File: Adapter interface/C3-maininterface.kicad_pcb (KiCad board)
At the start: 4 copper layers, 19.4 x 34.6 mm, 4 parts, among them J1 SFM-120-02-L-DH, J2 SFM-120-02-L-DH

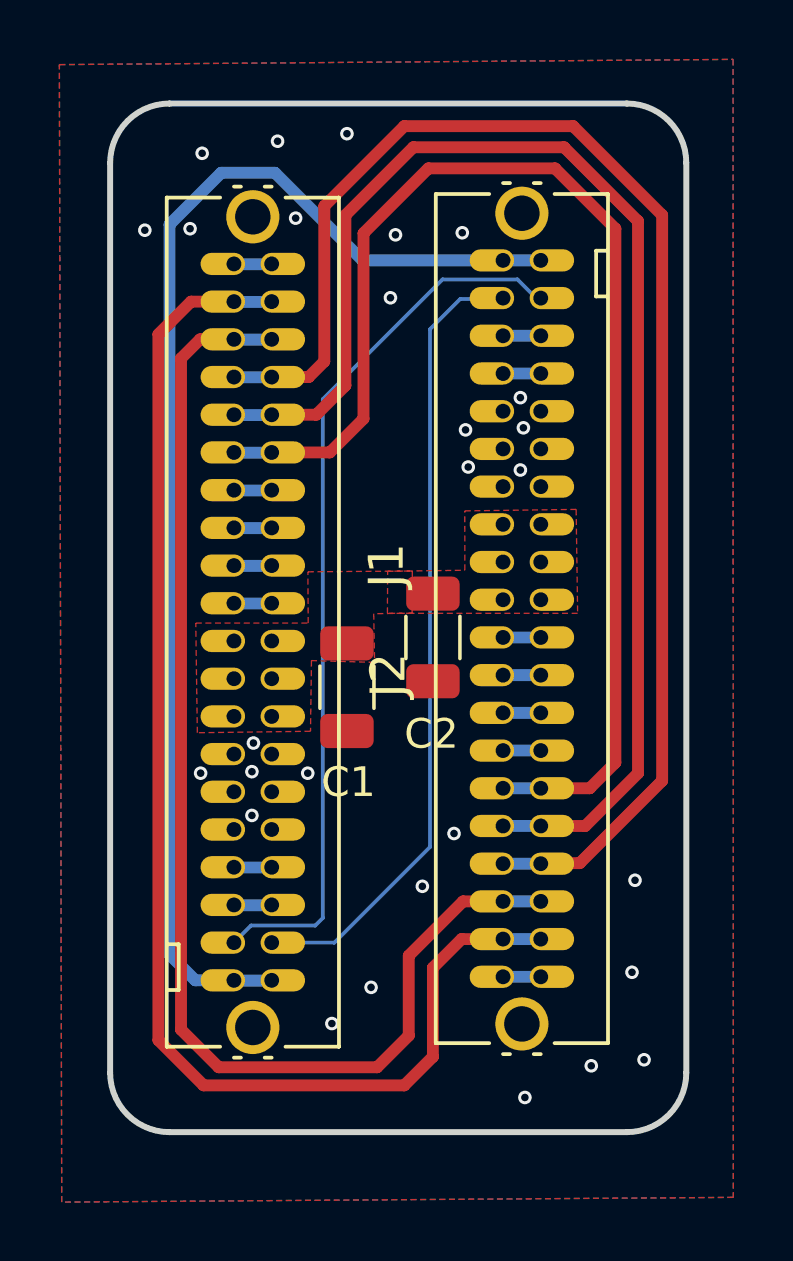
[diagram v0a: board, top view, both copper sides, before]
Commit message: New connectors
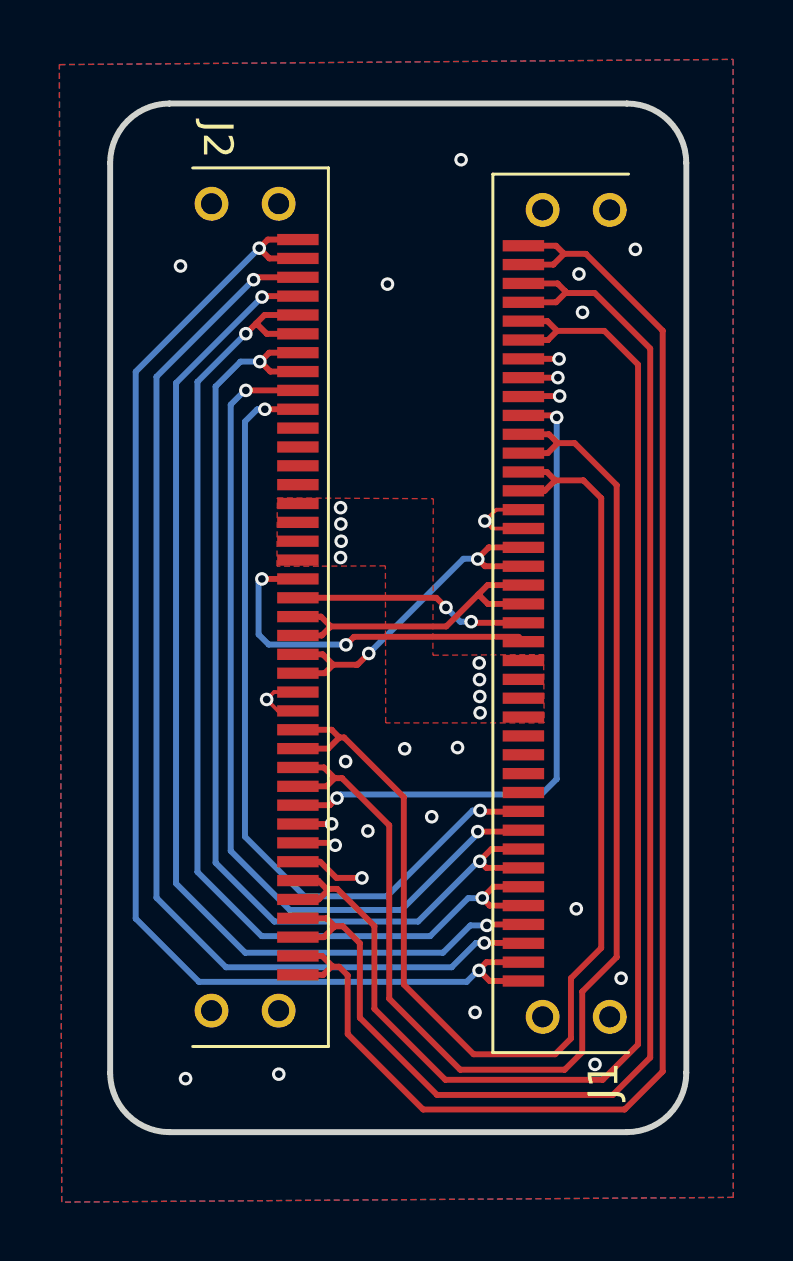
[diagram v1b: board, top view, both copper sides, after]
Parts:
- removed C1, C2: 10u 25V, Capacitor_SMD:C_1206_3216Metric
- J1, J2: footprint oresat-connectors:J-SAMTEC-SFM-120-X1-XXX-D -> oresat-connectors:SFM-120-02-X-DH
- moved J1 4.11 mm to (161.4, 85.6)
- moved J2 2.58 mm to (145.7, 85.4)
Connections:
- J1 pad 10: TURNSTILE-DEPLOY -> SPARE10
- J1 pad 21: VBUS -> SPARE21
- J1 pad 22: VBUS -> SPARE22
- J1 pad 31: GND -> SPARE31
- J1 pad 32: GND -> SPARE32
- J1 pad 7: HELICAL-DEPLOY -> SPARE07
- J1 pad 8: HELICAL-DEPLOY -> SPARE08
- J1 pad 9: TURNSTILE-DEPLOY -> SPARE09
- J2 pad 10: TURNSTILE-DEPLOY -> SPARE10
- J2 pad 21: VBUS -> SPARE21
- J2 pad 22: VBUS -> SPARE22
- J2 pad 31: GND -> SPARE31
- J2 pad 32: GND -> SPARE32
- J2 pad 7: HELICAL-DEPLOY -> SPARE07
- J2 pad 8: HELICAL-DEPLOY -> SPARE08
- J2 pad 9: TURNSTILE-DEPLOY -> SPARE09
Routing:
- net HELICAL-DEPLOY: track 47.8 -> 0.00 mm
- net TURNSTILE-DEPLOY: track 45.6 -> 0.00 mm
- net SPARE07: track 0.00 -> 29.7 mm, vias 0 -> 2
- net SPARE32: track 0.00 -> 29.3 mm, vias 0 -> 2
- net SPARE31: track 0.00 -> 27.4 mm, vias 0 -> 2
- net SPARE08: track 0.00 -> 27.0 mm, vias 0 -> 2
- net SPARE09: track 0.00 -> 24.2 mm, vias 0 -> 2
- net CAN2_H: track 34.8 -> 12.3 mm, vias 0 -> 2
- net SPARE10: track 0.00 -> 22.4 mm, vias 0 -> 2
- net CAN2_L: track 31.9 -> 11.2 mm
- net SPARE22: track 0.00 -> 12.4 mm, vias 0 -> 2
- net CAN1_H: track 24.7 -> 34.5 mm, vias 0 -> 2
- net C3-UART-TX: track 27.0 -> 35.2 mm, vias 0 -> 2
- net SPARE21: track 0.00 -> 7.95 mm, vias 0 -> 2
- net C3-UART-RX: track 30.1 -> 37.4 mm, vias 0 -> 2
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- added copper zone on In2.Cu, net VBUS
